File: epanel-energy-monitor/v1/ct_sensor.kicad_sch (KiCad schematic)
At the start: 8 parts, among them J19 Screw_Terminal_01x02

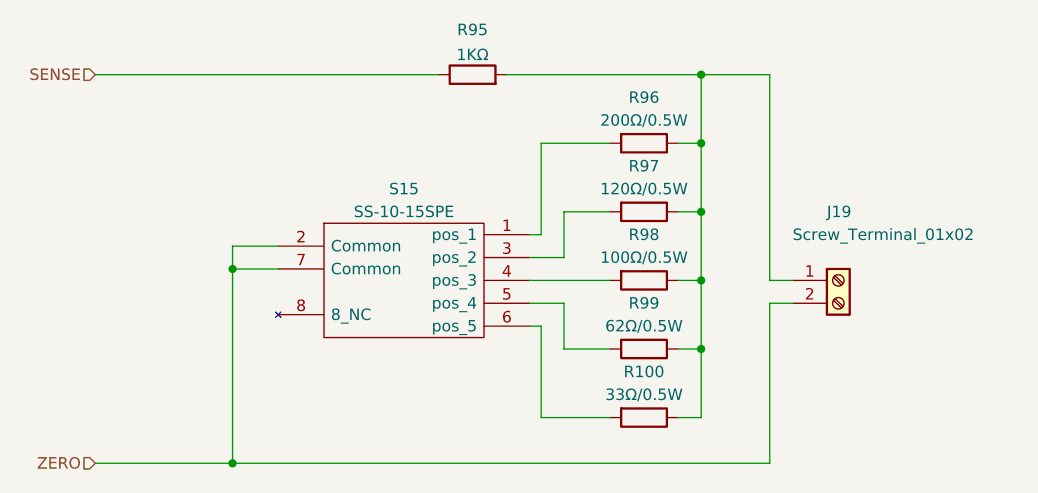
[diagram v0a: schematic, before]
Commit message: wip energy pcb
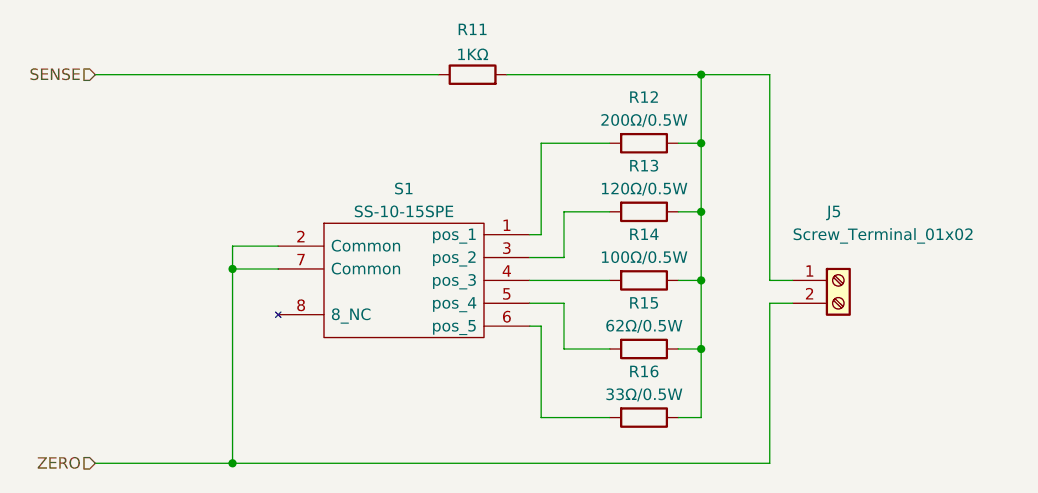
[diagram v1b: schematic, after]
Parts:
- renumbered J19 to J5, R95 to R11, R96 to R12, R97 to R13, R98 to R14, R99 to R15, R100 to R16, S15 to S1
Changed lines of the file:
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@@
   (symbol (lib_id "Device:R") (at 187.96 68.58 270)
     (in_bom yes) (on_board yes)
-    (property "Reference" "R97" (id 0) (at 187.96 63.5 90))
+    (property "Reference" "R13" (id 0) (at 187.96 63.5 90))
     (property "Value" "120Ω/0.5W" (id 1) (at 187.96 66.04 90))
     (property "Footprint" "Resistor_SMD:R_0805_2012Metric" (id 2) (at 187.96 66.802 90)
@@
   (symbol (lib_id "Device:R") (at 187.96 83.82 270)
     (in_bom yes) (on_board yes)
-    (property "Reference" "R99" (id 0) (at 187.96 78.74 90))
+    (property "Reference" "R15" (id 0) (at 187.96 78.74 90))
     (property "Value" "62Ω/0.5W" (id 1) (at 187.96 81.28 90))
     (property "Footprint" "Resistor_SMD:R_0805_2012Metric" (id 2) (at 187.96 82.042 90)
@@
   (symbol (lib_id "Device:R") (at 168.91 53.34 90)
     (in_bom yes) (on_board yes) (fields_autoplaced)
-    (property "Reference" "R95" (id 0) (at 168.91 48.3575 90))
+    (property "Reference" "R11" (id 0) (at 168.91 48.3575 90))
     (property "Value" "1KΩ" (id 1) (at 168.91 51.1326 90))
     (property "Footprint" "Resistor_SMD:R_0603_1608Metric" (id 2) (at 168.91 55.118 90)
@@
   (symbol (lib_id "Connector:Screw_Terminal_01x02") (at 209.55 76.2 0)
     (in_bom yes) (on_board yes)
-    (property "Reference" "J19" (id 0) (at 208.28 68.58 0)
+    (property "Reference" "J5" (id 0) (at 208.28 68.58 0)
       (effects (font (size 1.27 1.27)) (justify left))
     )
@@
   (symbol (lib_id "Device:R") (at 187.96 60.96 270)
     (in_bom yes) (on_board yes)
-    (property "Reference" "R96" (id 0) (at 187.96 55.88 90))
+    (property "Reference" "R12" (id 0) (at 187.96 55.88 90))
     (property "Value" "200Ω/0.5W" (id 1) (at 187.96 58.42 90))
     (property "Footprint" "Resistor_SMD:R_0805_2012Metric" (id 2) (at 187.96 59.182 90)
@@
   (symbol (lib_id "mylife-symbols:SS-10-15SPE") (at 161.29 76.2 0)
     (in_bom yes) (on_board yes)
-    (property "Reference" "S15" (id 0) (at 161.29 66.04 0))
+    (property "Reference" "S1" (id 0) (at 161.29 66.04 0))
     (property "Value" "SS-10-15SPE" (id 1) (at 161.29 68.58 0))
     (property "Footprint" "mylife-footprints:RS PRO SS-10-15SPE" (id 2) (at 185.42 73.66 0)
@@
   (symbol (lib_id "Device:R") (at 187.96 91.44 270)
     (in_bom yes) (on_board yes)
-    (property "Reference" "R100" (id 0) (at 187.96 86.36 90))
+    (property "Reference" "R16" (id 0) (at 187.96 86.36 90))
     (property "Value" "33Ω/0.5W" (id 1) (at 187.96 88.9 90))
     (property "Footprint" "Resistor_SMD:R_0805_2012Metric" (id 2) (at 187.96 89.662 90)
@@
   (symbol (lib_id "Device:R") (at 187.96 76.2 270)
     (in_bom yes) (on_board yes)
-    (property "Reference" "R98" (id 0) (at 187.96 71.12 90))
+    (property "Reference" "R14" (id 0) (at 187.96 71.12 90))
     (property "Value" "100Ω/0.5W" (id 1) (at 187.96 73.66 90))
     (property "Footprint" "Resistor_SMD:R_0805_2012Metric" (id 2) (at 187.96 74.422 90)

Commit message: wip energy pcb
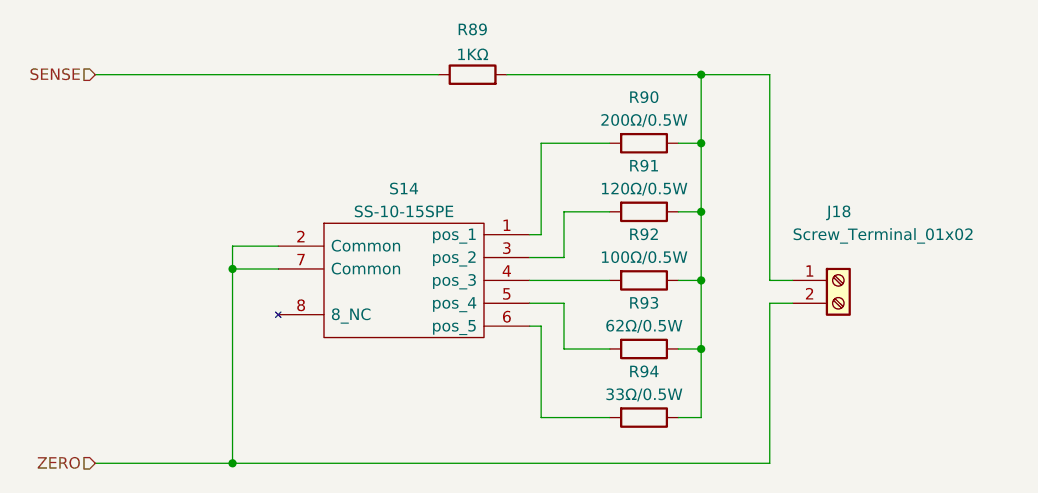
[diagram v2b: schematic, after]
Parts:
- renumbered J5 to J18, R11 to R89, R12 to R90, R13 to R91, R14 to R92, R15 to R93, R16 to R94, S1 to S14
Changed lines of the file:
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@@
   (symbol (lib_id "Device:R") (at 187.96 68.58 270)
     (in_bom yes) (on_board yes)
-    (property "Reference" "R13" (id 0) (at 187.96 63.5 90))
+    (property "Reference" "R91" (id 0) (at 187.96 63.5 90))
     (property "Value" "120Ω/0.5W" (id 1) (at 187.96 66.04 90))
     (property "Footprint" "Resistor_SMD:R_0805_2012Metric" (id 2) (at 187.96 66.802 90)
@@
   (symbol (lib_id "Device:R") (at 187.96 83.82 270)
     (in_bom yes) (on_board yes)
-    (property "Reference" "R15" (id 0) (at 187.96 78.74 90))
+    (property "Reference" "R93" (id 0) (at 187.96 78.74 90))
     (property "Value" "62Ω/0.5W" (id 1) (at 187.96 81.28 90))
     (property "Footprint" "Resistor_SMD:R_0805_2012Metric" (id 2) (at 187.96 82.042 90)
@@
   (symbol (lib_id "Device:R") (at 168.91 53.34 90)
     (in_bom yes) (on_board yes) (fields_autoplaced)
-    (property "Reference" "R11" (id 0) (at 168.91 48.3575 90))
+    (property "Reference" "R89" (id 0) (at 168.91 48.3575 90))
     (property "Value" "1KΩ" (id 1) (at 168.91 51.1326 90))
     (property "Footprint" "Resistor_SMD:R_0603_1608Metric" (id 2) (at 168.91 55.118 90)
@@
   (symbol (lib_id "Connector:Screw_Terminal_01x02") (at 209.55 76.2 0)
     (in_bom yes) (on_board yes)
-    (property "Reference" "J5" (id 0) (at 208.28 68.58 0)
+    (property "Reference" "J18" (id 0) (at 208.28 68.58 0)
       (effects (font (size 1.27 1.27)) (justify left))
     )
@@
   (symbol (lib_id "Device:R") (at 187.96 60.96 270)
     (in_bom yes) (on_board yes)
-    (property "Reference" "R12" (id 0) (at 187.96 55.88 90))
+    (property "Reference" "R90" (id 0) (at 187.96 55.88 90))
     (property "Value" "200Ω/0.5W" (id 1) (at 187.96 58.42 90))
     (property "Footprint" "Resistor_SMD:R_0805_2012Metric" (id 2) (at 187.96 59.182 90)
@@
   (symbol (lib_id "mylife-symbols:SS-10-15SPE") (at 161.29 76.2 0)
     (in_bom yes) (on_board yes)
-    (property "Reference" "S1" (id 0) (at 161.29 66.04 0))
+    (property "Reference" "S14" (id 0) (at 161.29 66.04 0))
     (property "Value" "SS-10-15SPE" (id 1) (at 161.29 68.58 0))
     (property "Footprint" "mylife-footprints:RS PRO SS-10-15SPE" (id 2) (at 185.42 73.66 0)
@@
   (symbol (lib_id "Device:R") (at 187.96 91.44 270)
     (in_bom yes) (on_board yes)
-    (property "Reference" "R16" (id 0) (at 187.96 86.36 90))
+    (property "Reference" "R94" (id 0) (at 187.96 86.36 90))
     (property "Value" "33Ω/0.5W" (id 1) (at 187.96 88.9 90))
     (property "Footprint" "Resistor_SMD:R_0805_2012Metric" (id 2) (at 187.96 89.662 90)
@@
   (symbol (lib_id "Device:R") (at 187.96 76.2 270)
     (in_bom yes) (on_board yes)
-    (property "Reference" "R14" (id 0) (at 187.96 71.12 90))
+    (property "Reference" "R92" (id 0) (at 187.96 71.12 90))
     (property "Value" "100Ω/0.5W" (id 1) (at 187.96 73.66 90))
     (property "Footprint" "Resistor_SMD:R_0805_2012Metric" (id 2) (at 187.96 74.422 90)
